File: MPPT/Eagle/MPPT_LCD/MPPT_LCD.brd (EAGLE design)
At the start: 102 x 82 mm, 12 parts, among them IC1 MCP23017SP, U1 ARDUINOR3LONGHEADERATBOTTOM, X2 HD44780LCD

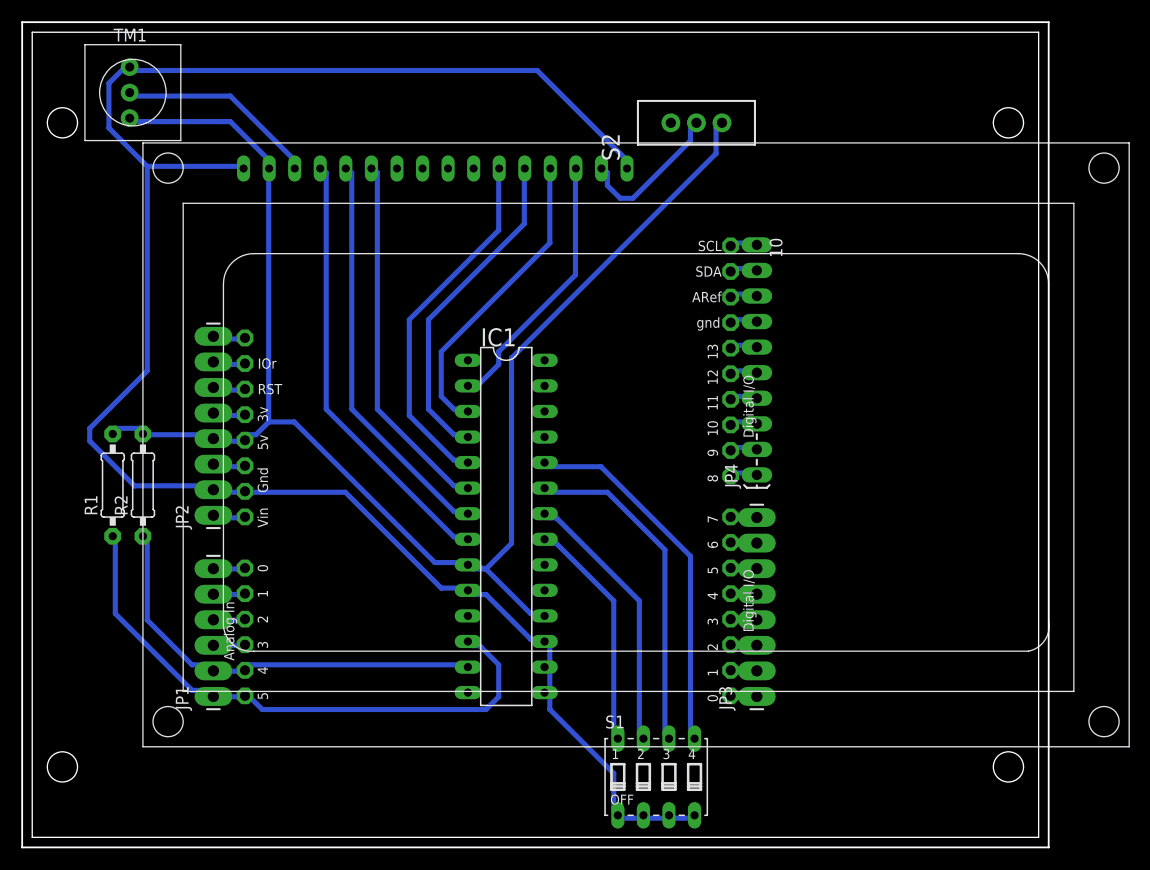
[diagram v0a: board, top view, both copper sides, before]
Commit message: pin headers
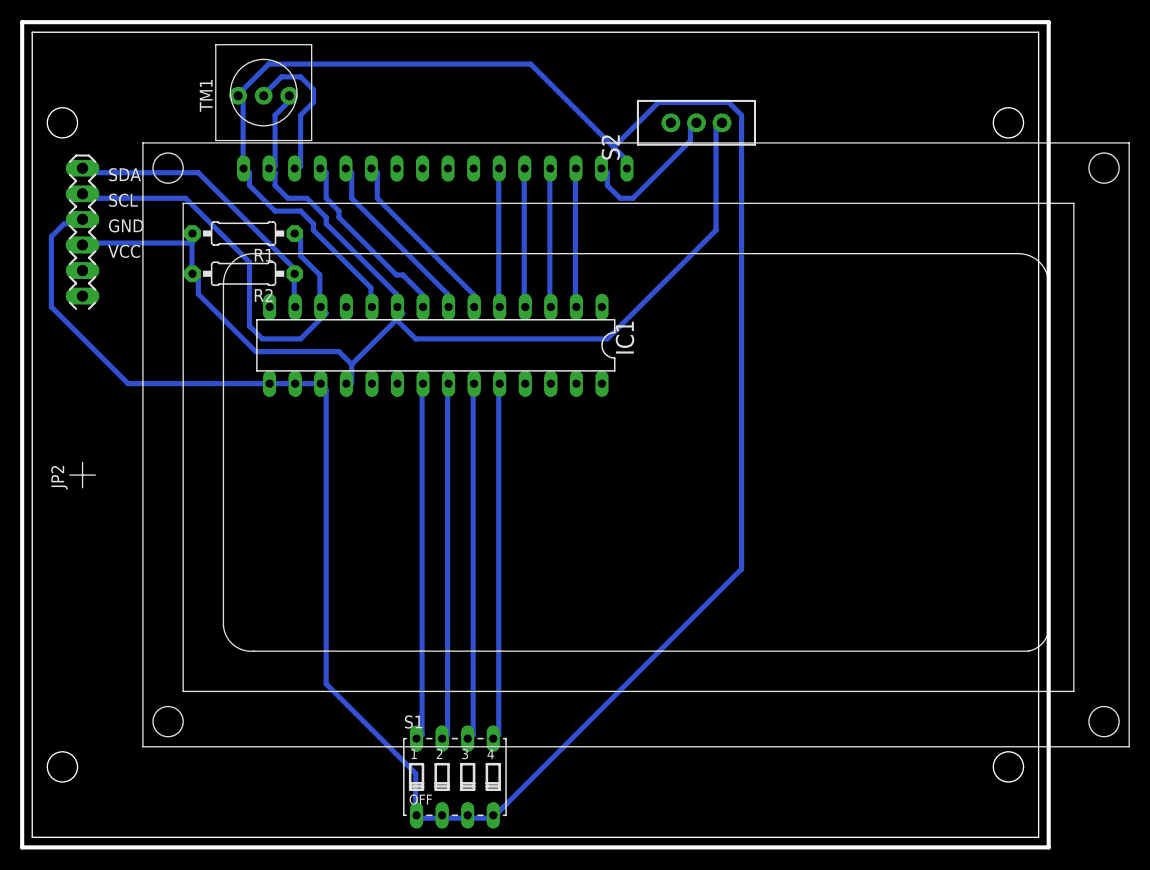
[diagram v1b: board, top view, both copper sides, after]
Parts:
- removed JP1: (no value), tmb_connectors:1X06_LONGPADS
- removed JP3: (no value), tmb_connectors:1X08_LONGPADS
- removed JP4: (no value), tmb_connectors:1X10_LONGPADS
- removed U1: ARDUINOR3LONGHEADERATBOTTOM, tmb_boards:ARDUINOR3-BPLACE_TURNED
- JP2: device tmb_connectors:1X08_LONGPADS -> tmb_connectors:M06_MPPT_DATA
- moved R1 28.2 mm to (21.0, 60.0), turned to 180 degrees
- moved R2 23.3 mm to (21.0, 56.0), turned to 180 degrees
- moved S1 20.0 mm to (42.0, 6.00)
- moved IC1 19.3 mm to (40.1, 48.9), turned to 180 degrees
- moved JP2 13.6 mm to (5.00, 36.0)
- moved TM1 13.0 mm to (23.0, 74.0), turned to 0 degrees
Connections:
- removed net N$1: JP4.7, U1.GND
- removed net N$13: JP3.4, U1.D3
- removed net N$14: JP1.3, U1.A3
- removed net N$15: JP1.4, U1.A2
- removed net N$16: JP1.5, U1.A1
- removed net N$17: JP1.6, U1.A0
- removed net N$18: JP2.1, U1.VIN
- removed net N$20: JP2.3, U1.GND2
- removed net N$22: JP2.5, U1.3V
- removed net N$23: JP2.6, U1.RESET
- removed net N$24: JP2.7, U1.IOREF
- removed net N$25: JP2.8, U1.RESERVED
- removed net N$26: JP3.1, U1.D0
- removed net N$27: JP3.2, U1.D1
- removed net N$28: JP3.3, U1.D2
- removed net N$29: JP3.5, U1.D4
- removed net N$30: JP3.6, U1.D5
- removed net N$31: JP3.7, U1.D6
- removed net N$32: JP3.8, U1.D7
- removed net N$33: JP4.1, U1.D8
- removed net N$34: JP4.2, U1.D9
- removed net N$35: JP4.3, U1.D10
- removed net N$36: JP4.4, U1.D11
- removed net N$37: JP4.5, U1.D12
- removed net N$38: JP4.6, U1.D13
- removed net N$40: JP4.8, U1.AREF
- removed net N$41: JP4.9, U1.SDA
- removed net N$42: JP4.10, U1.SCL
- net 5V: now also JP2.10; no longer JP2.4, U1.5V
- net GND: now also JP2.11; no longer JP2.2, U1.GND1
- net N$11: now also JP2.13; no longer JP1.2, U1.A4
- net N$12: now also JP2.12; no longer JP1.1, U1.A5
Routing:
- net GND: track 189.7 -> 263.9 mm
- net 5V: track 150.3 -> 124.5 mm
- net N$10: track 43.7 -> 18.5 mm
- net N$7: track 36.0 -> 13.9 mm
- net N$9: track 40.1 -> 18.1 mm
- net N$6: track 33.0 -> 13.9 mm
- net N$8: track 36.5 -> 18.1 mm
- net N$5: track 30.4 -> 13.9 mm
- net N$11: track 43.2 -> 29.3 mm
- net N$12: track 57.8 -> 44.5 mm
- net N$4: track 26.9 -> 13.9 mm
- net N$3: track 23.3 -> 35.6 mm
- net N$19: track 26.8 -> 35.6 mm
- net N$2: track 19.9 -> 15.1 mm
- net N$22: track 3.23 -> 0.00 mm
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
